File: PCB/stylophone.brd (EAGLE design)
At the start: 102.5 x 80 mm, 24 parts, among them IC2 LM358N

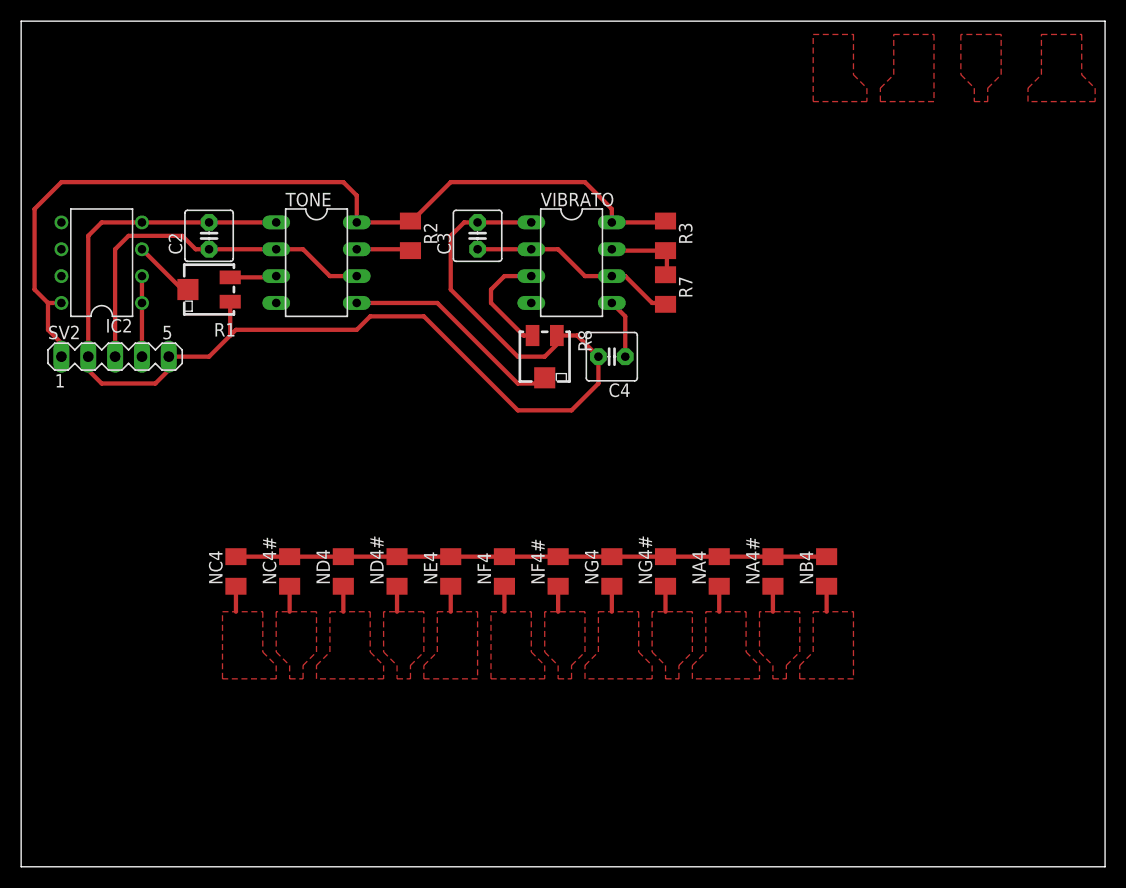
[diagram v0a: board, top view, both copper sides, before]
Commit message: almost done
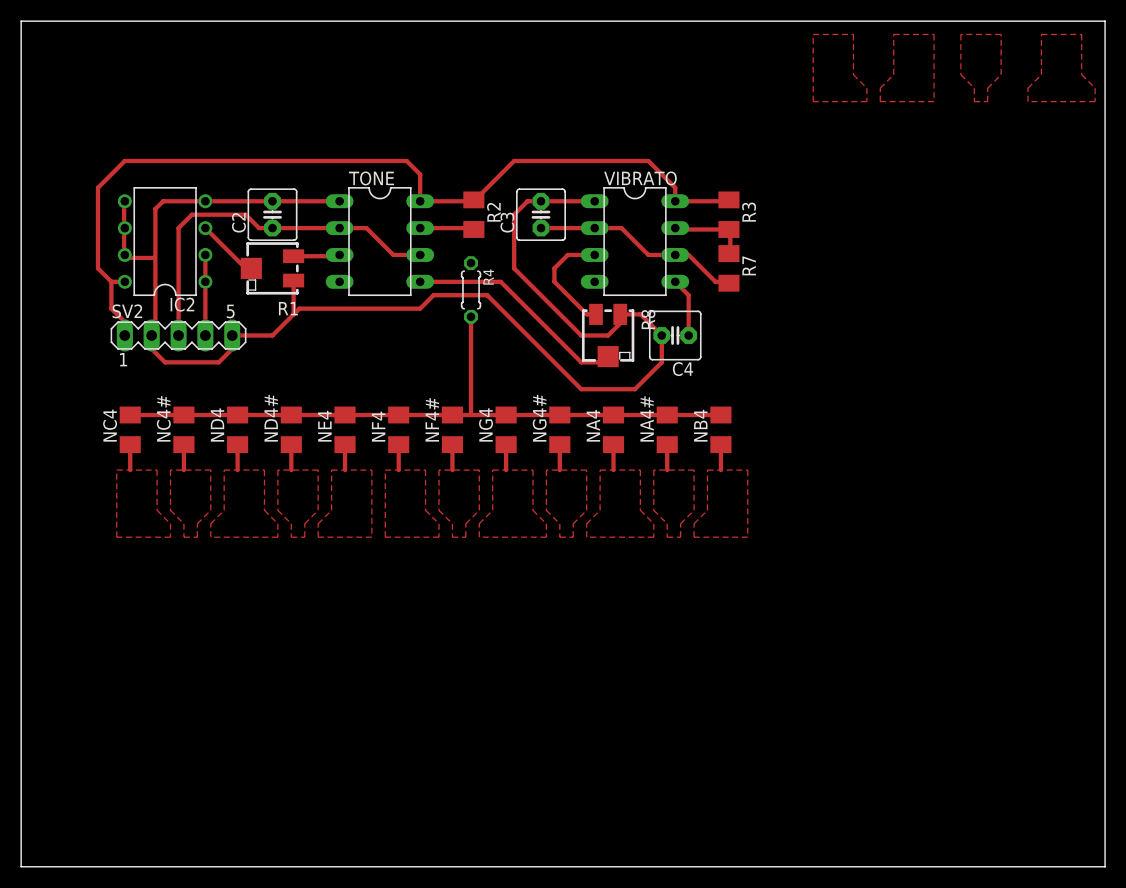
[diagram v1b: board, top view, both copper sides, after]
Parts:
- added R4: (no value), rcl:0204/5
- moved NA4 16.7 mm to (53.5, 41.3)
- moved NA4# 16.7 mm to (58.6, 41.3)
- moved NB4 16.7 mm to (63.7, 41.3)
- moved NC4 16.7 mm to (7.78, 41.3)
- moved NC4# 16.7 mm to (12.9, 41.3)
- moved ND4 16.7 mm to (17.9, 41.3)
- moved ND4# 16.7 mm to (23.0, 41.3)
- moved NE4 16.7 mm to (28.1, 41.3)
- moved NF4 16.7 mm to (33.2, 41.3)
- moved NF4# 16.7 mm to (38.3, 41.3)
- moved NG4 16.7 mm to (43.3, 41.3)
- moved NG4# 16.7 mm to (48.4, 41.3)
- moved C3 6.32 mm to (46.6, 61.7)
- moved C4 6.32 mm to (59.3, 50.3)
- moved IC2 6.32 mm to (11.1, 59.1)
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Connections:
- new net KEYBOARD: NA4#.2, NA4.2, NB4.2, NC4#.2, NC4.2, ND4#.2, ND4.2, NE4.2, NF4#.2, NF4.2, NG4#.2, NG4.2, R4.2
- net NOTE: now also R4.1; no longer NA4#.2, NA4.2, NB4.2, NC4#.2, NC4.2, ND4#.2, ND4.2, NE4.2, NF4#.2, NF4.2, NG4#.2, NG4.2
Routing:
- net KEYBOARD: track 0.00 -> 65.4 mm
- net NOTE: track 61.3 -> 5.21 mm
- net N$21: track 0.00 -> 8.00 mm
- net GND: track 125.7 -> 126.4 mm

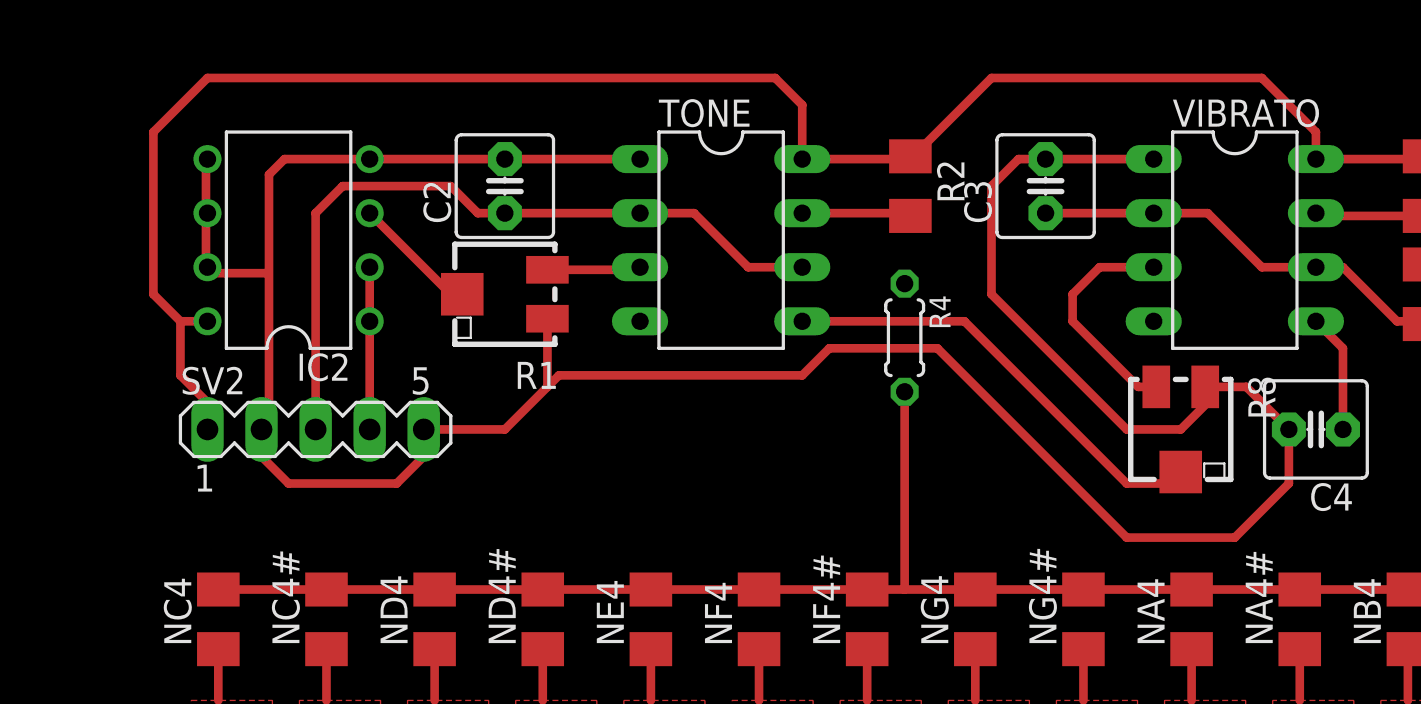
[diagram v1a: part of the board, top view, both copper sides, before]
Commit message: pots
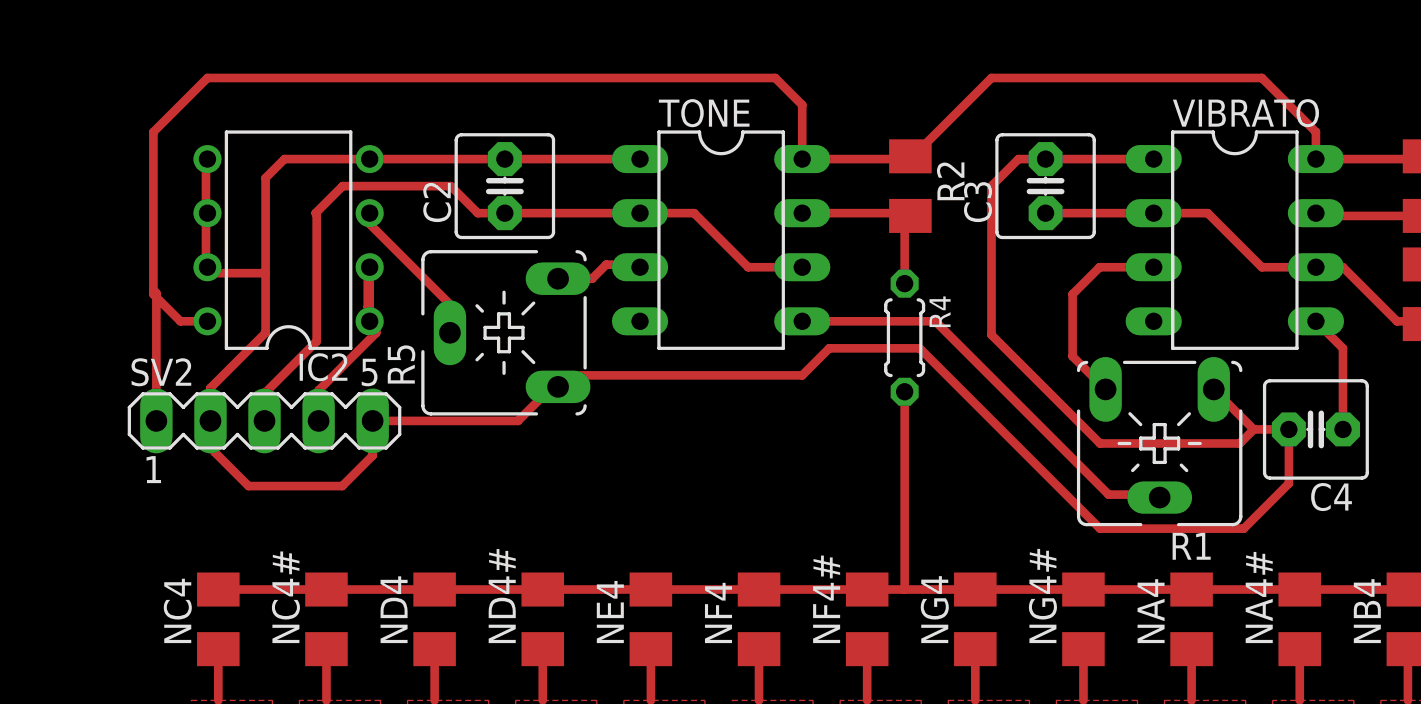
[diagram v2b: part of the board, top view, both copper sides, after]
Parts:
- removed R8: (no value), resistor:RTRIM5X
- added R5: (no value), pot:CA6V
- R1: device resistor:RTRIM5X -> pot:CA6V
- moved R1 31.5 mm to (52.0, 49.6), turned to 180 degrees
- moved SV2 2.43 mm to (9.95, 50.7)
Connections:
- net GND: now also R1.A, R5.A; no longer R1.1, R8.1
- net N$2: now also R1.E; no longer R8.3
- net N$5: now also R5.S; no longer R1.2
- net TONE: now also R5.E; no longer R1.3
- net VIBRATO: now also R1.S; no longer R8.2
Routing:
- net OUTPUT: track 7.62 -> 11.1 mm
- net NOTE: track 5.21 -> 8.50 mm
- net GND: track 126.4 -> 128.0 mm
- net N$5: track 5.93 -> 7.30 mm
- net N$2: track 10.8 -> 9.45 mm
- net VIBRATO: track 21.2 -> 20.2 mm
- net STYLUS: track 33.9 -> 34.5 mm
- net VCC: track 84.2 -> 84.8 mm
